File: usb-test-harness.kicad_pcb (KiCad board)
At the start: 4 copper layers, 98 x 85 mm, 92 parts, among them J1 Conn_01x06, J10 USB_A_DUAL, J4 USB_A (female down), J5 Conn_01x03_Male, J6 USB_A_DUAL, J7 USB_A_DUAL, J8 USB_A male UP, J9 USB_B_Micro (up), U1 2k i2c eeprom, U10 NUP4202, U11 NUP4202, U12 NUP4202, U2 SE5120ST33, U3 USB2517, U4 APL3511C, U5 APL3511C, U6 APL3511C, U7 APL3511C, U8 APL3511C, U9 APL3511C, Y1 24MHz

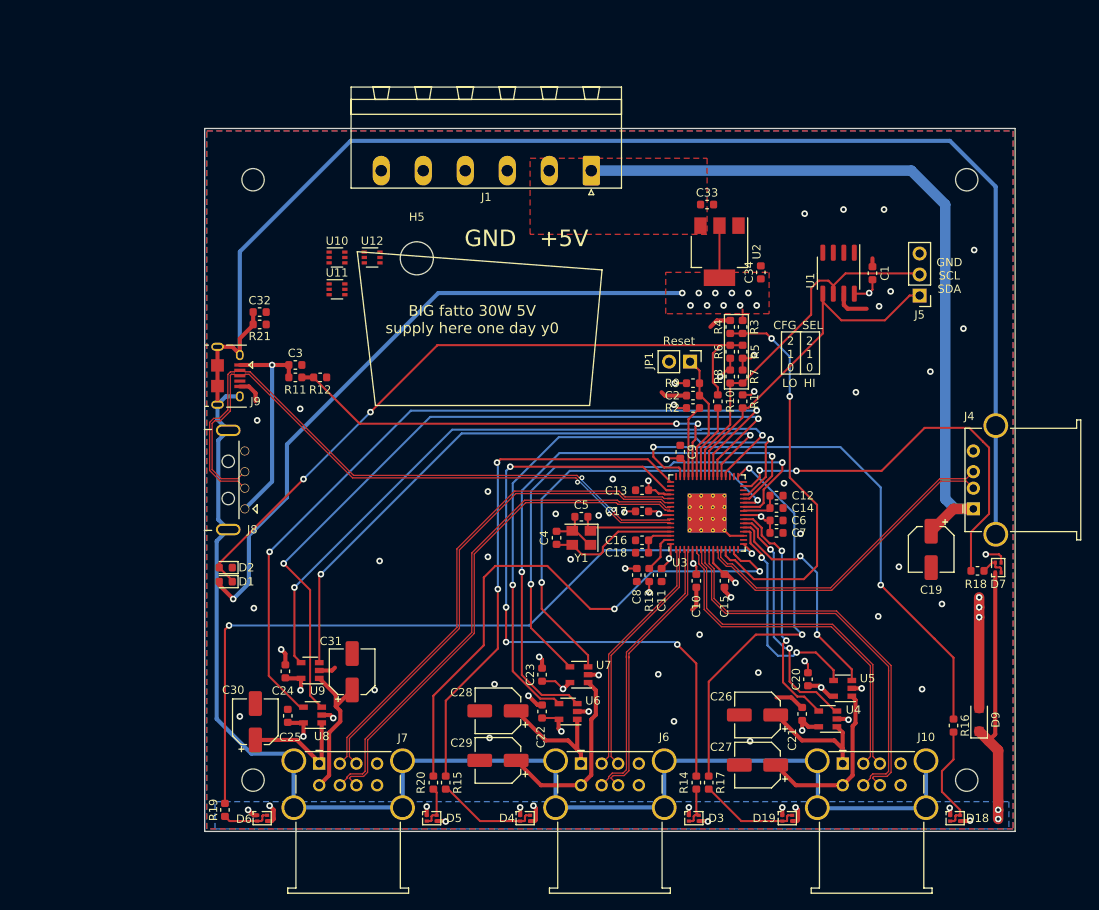
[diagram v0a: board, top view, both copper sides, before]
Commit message: Updated "finished" for new bud cu-388 box
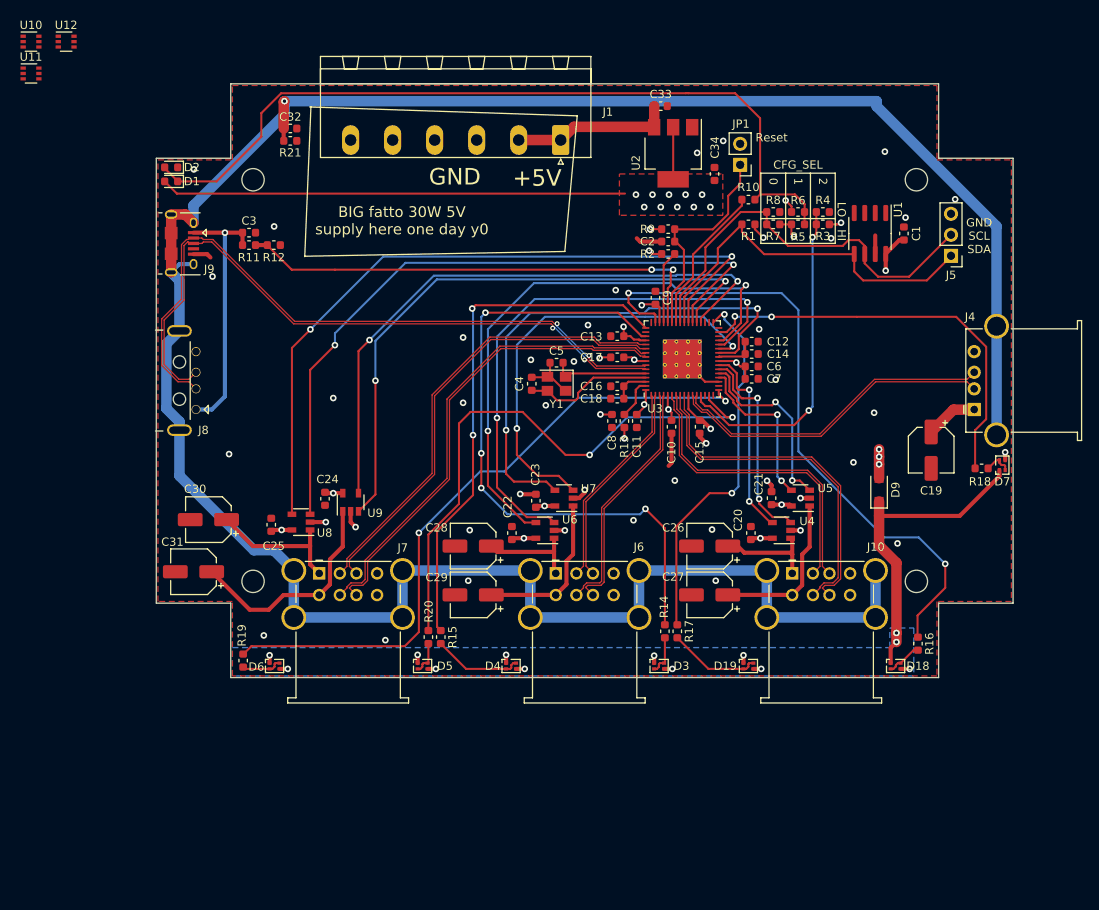
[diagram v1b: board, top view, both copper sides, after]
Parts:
- removed H5: MountingHole, MountingHole:MountingHole_4mm
- moved D1 48.8 mm to (95.2, 57.0)
- moved D2 48.8 mm to (95.2, 55.3)
- moved U10 45.3 mm to (78.2, 40.1)
- moved U12 45.3 mm to (82.5, 40.1)
- moved U11 45.3 mm to (78.2, 44.0)
- moved D9 30.3 mm to (180.8, 94.3)
- moved C21 26.4 mm to (167.8, 95.3)
- moved C30 25.1 mm to (99.7, 97.9), turned to 180 degrees
- moved H4 24.8 mm to (185.3, 105.4)
- moved R10 24.7 mm to (165.0, 59.2), turned to 180 degrees
- moved JP1 24.6 mm to (164.0, 55.0), turned to 180 degrees
- moved H2 24.0 mm to (105.1, 105.4)
- moved J10 23.8 mm to (170.3, 104.4)
- moved U5 23.6 mm to (171.3, 95.3)
- moved U4 23.5 mm to (169.0, 99.2)
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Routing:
- net +5V: track 112.0 -> 41.0 mm
- net +3V3: track 141.1 -> 109.9 mm
- net GNDPWR: track 334.6 -> 306.7 mm, vias 0 -> 1
- net GND: track 67.5 -> 47.1 mm, vias 54 -> 50
- net /upstream-config-leds/CFG_SEL1: track 83.3 -> 98.5 mm, vias 2 -> 0
- net /upstream-config-leds/LED_A3: track 67.1 -> 78.1 mm
- net /upstream-config-leds/~RESET: track 15.5 -> 26.2 mm
- net /upstream-config-leds/LED_A6: track 90.4 -> 80.1 mm
- net /downstream-port-power/OC5: track 93.2 -> 84.0 mm
- net /downstream-port-power/VBUS6: track 17.8 -> 26.9 mm
- net /upstream-config-leds/CFG_SEL1_A: track 9.15 -> 18.2 mm
- net /upstream-config-leds/LA_3-1: track 13.3 -> 4.34 mm
- net /downstream-port-power/EN5: track 97.0 -> 88.1 mm
- net /upstream-config-leds/CFG_SEL2: track 48.7 -> 40.1 mm
- net /downstream-port-power/EN6: track 81.1 -> 74.0 mm
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- removed copper zone on F.Cu, net +5V
- removed copper zone on B.Cu, net GND
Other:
- board size 98 x 85 mm -> 103.6 x 71.8 mm
- board text added: "0"
- board text added: "1"
- board text added: "2"
- board text removed: "2 1 0"
